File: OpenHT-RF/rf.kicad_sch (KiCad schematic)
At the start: 42 parts, among them J501 EMPCB.CSMAFSTJ.A, J502 Conn_01x02, J503 Conn_01x02, J504 MS300-10F, J505 MS300-10C, SW501 RFSW8008, U501 AT86RF215, X501 ECS-TXO-20CSMV

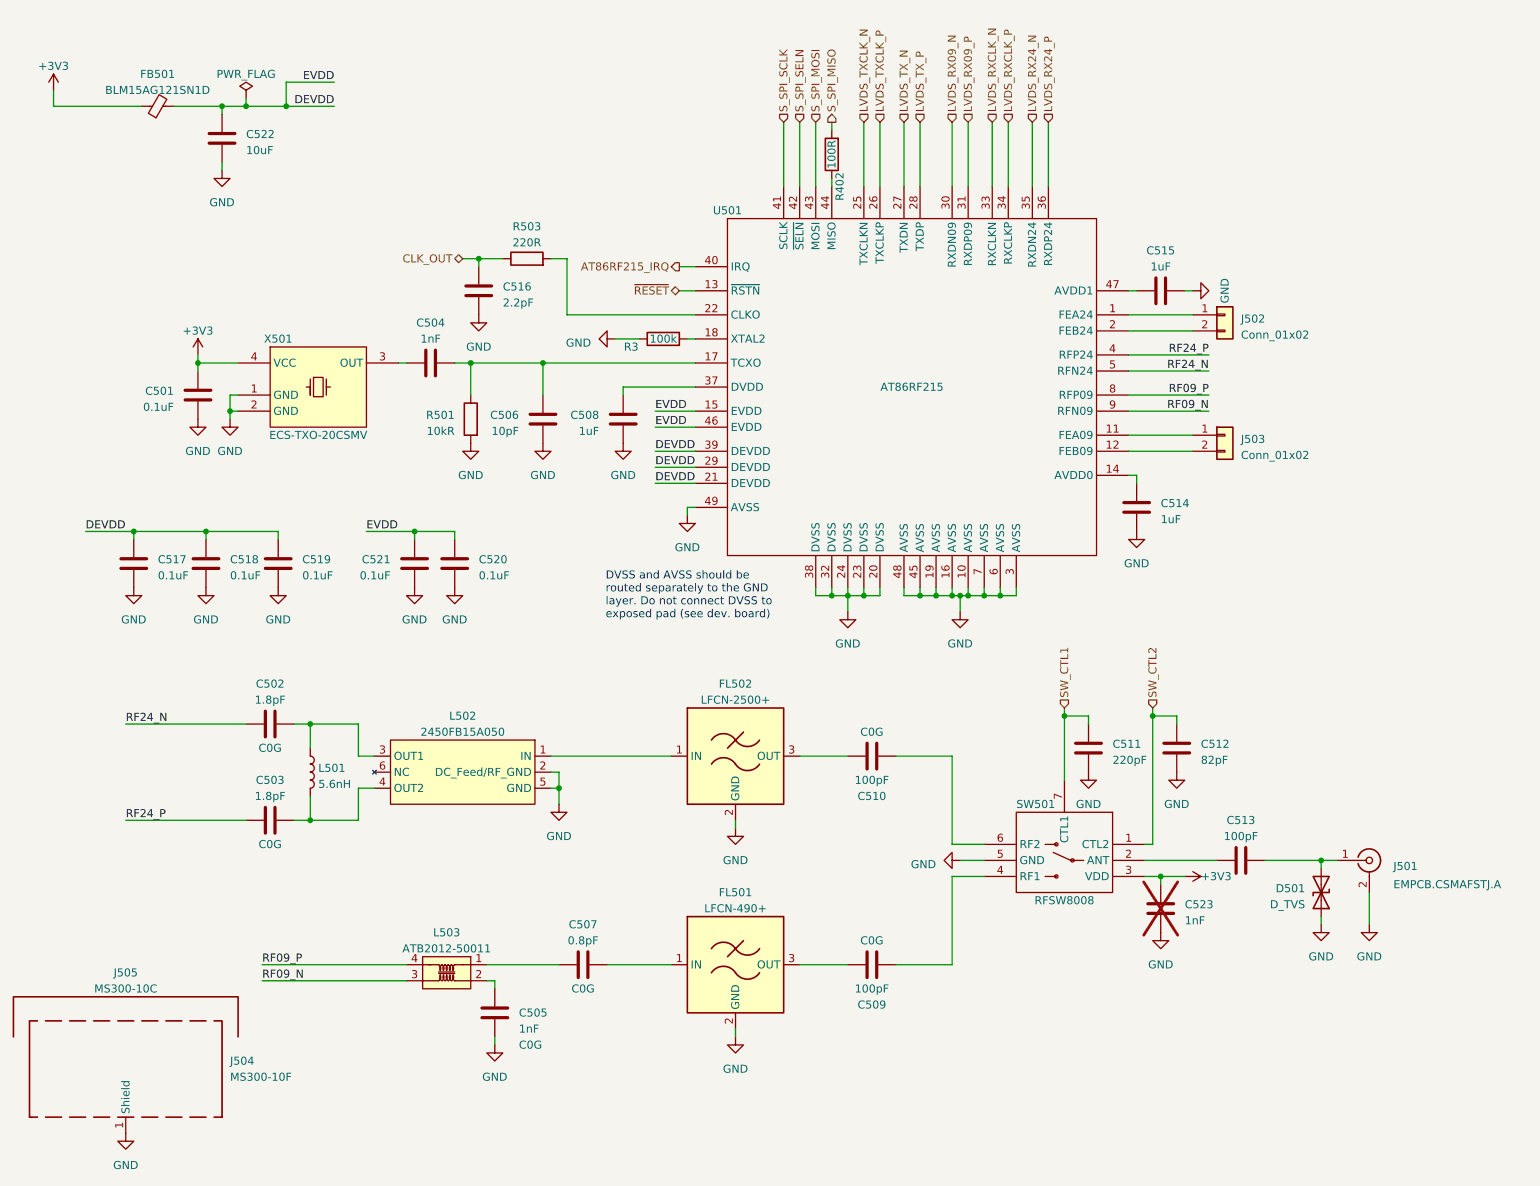
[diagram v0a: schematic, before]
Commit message: Completed components values
Completed dielectric, rated voltage, tolerance, MPN
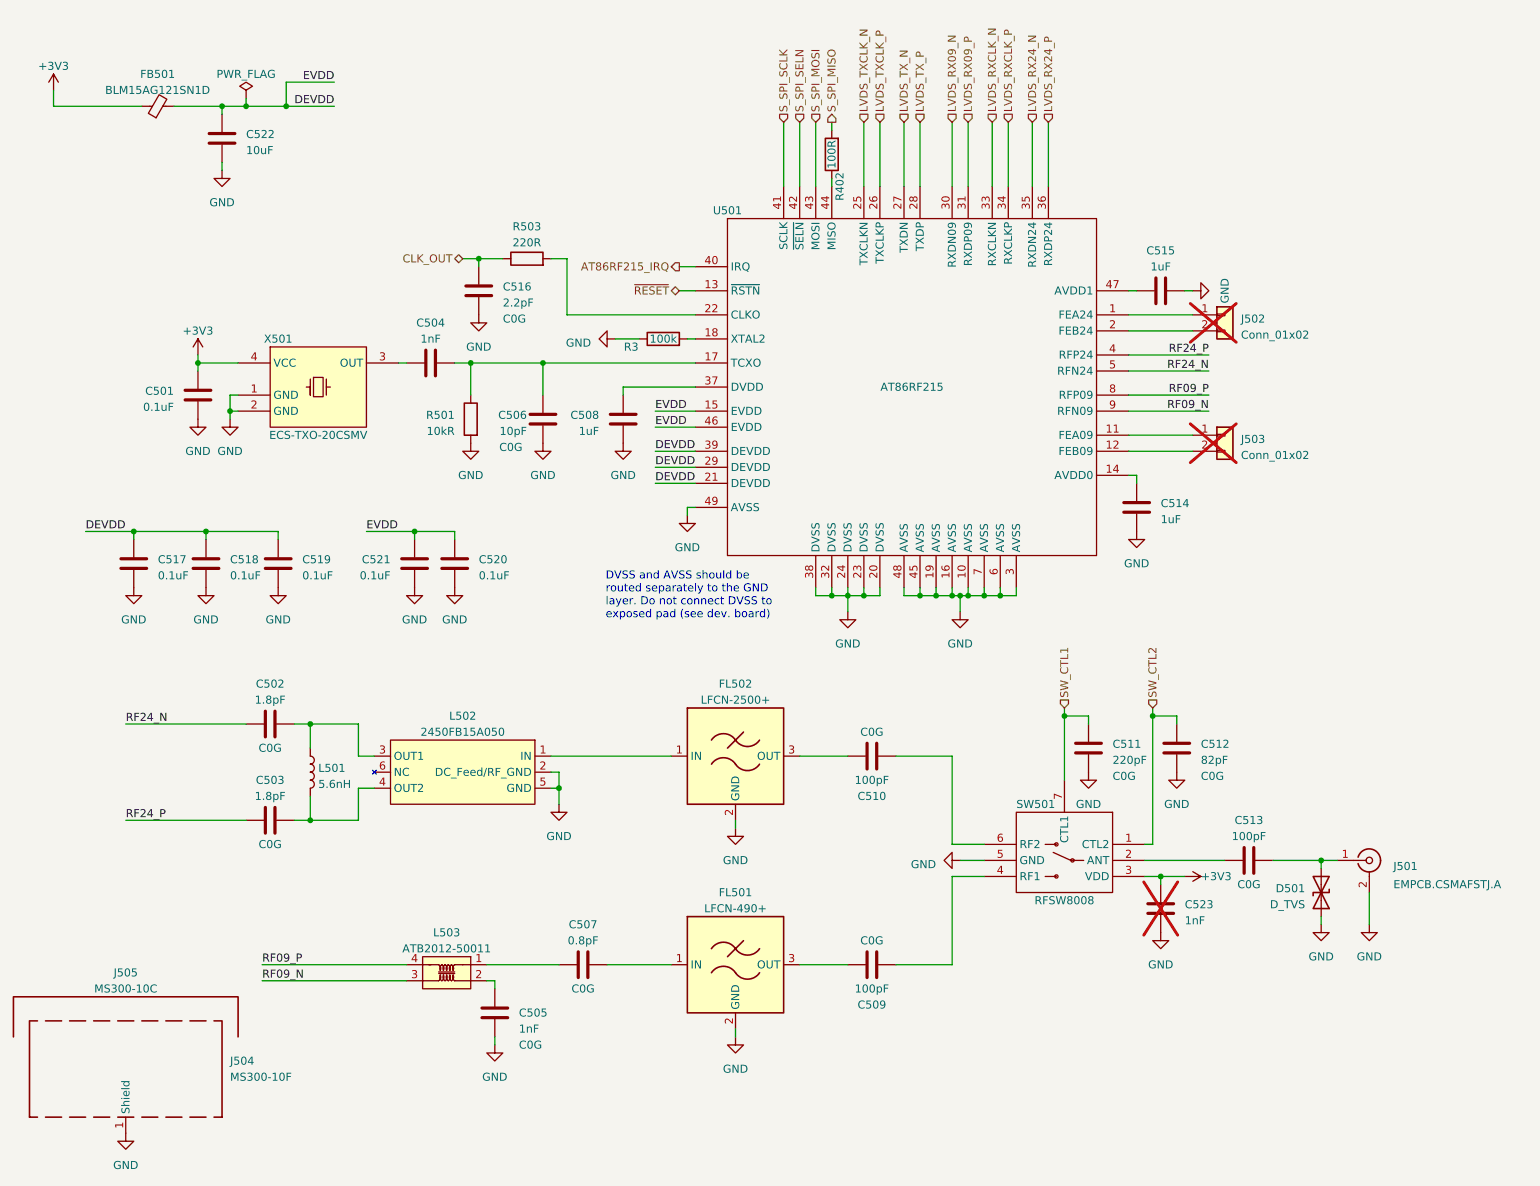
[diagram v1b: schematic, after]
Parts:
- C506, C511, C512, C513, C516: Dielectric (none) -> C0G
- J502, J503: now not fitted
- J505: Manual_Placement (none) -> 1
- R3, R402, R501, R503: Tolerance (none) -> 1%
- SW501: MPN (none) -> RFSW8008TR7
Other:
- moved on the sheet: C513
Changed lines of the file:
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@@
     (stroke (width 0) (type default))
   )
-  (wire (pts (xy 215.9 146.05) (xy 224.79 146.05))
+  (wire (pts (xy 217.17 146.05) (xy 224.79 146.05))
     (stroke (width 0) (type default))
   )
@@
     (stroke (width 0) (type default))
   )
-  (wire (pts (xy 196.85 146.05) (xy 208.28 146.05))
+  (wire (pts (xy 196.85 146.05) (xy 209.55 146.05))
     (stroke (width 0) (type default))
   )
@@
     )
   )
-  (netclass_flag "" (length 2.54) (shape round) (at 217.17 146.05 0) (fields_autoplaced)
+  (netclass_flag "" (length 2.54) (shape round) (at 218.44 146.05 0) (fields_autoplaced)
     (effects (font (size 1.27 1.27)) (justify left bottom))
-    (property "Netclass" "50Ohm" (at 217.8685 143.51 0)
+    (property "Netclass" "50Ohm" (at 219.1385 143.51 0)
       (effects (font (size 1.27 1.27) italic) (justify left))
     )
@@
     )
     (property "MPN" "MS300-10C" (at 35.56 171.45 0)
+      (effects (font (size 1.27 1.27)) hide)
+    )
+    (property "Manual_Placement" "1" (at 35.56 171.45 0)
       (effects (font (size 1.27 1.27)) hide)
     )
@@
       (effects (font (size 1.27 1.27)) hide)
     )
+    (property "Tolerance" "1%" (at 90.17 76.2 0)
+      (effects (font (size 1.27 1.27)) hide)
+    )
     (pin "1")
     (pin "2")
@@
   )
   (symbol (lib_id "Device:C") (at 187.96 128.27 0) (unit 1)
-    (in_bom yes) (on_board yes) (dnp no) (fields_autoplaced)
+    (in_bom yes) (on_board yes) (dnp no)
     (property "Reference" "C511" (at 191.77 127.635 0)
       (effects (font (size 1.27 1.27)) (justify left))
@@
       (effects (font (size 1.27 1.27)) hide)
     )
+    (property "Dielectric" "C0G" (at 191.77 132.715 0)
+      (effects (font (size 1.27 1.27)) (justify left))
+    )
     (pin "1")
     (pin "2")
@@
   )
   (symbol (lib_id "Device:C") (at 201.93 128.27 0) (unit 1)
-    (in_bom yes) (on_board yes) (dnp no) (fields_autoplaced)
+    (in_bom yes) (on_board yes) (dnp no)
     (property "Reference" "C512" (at 205.74 127.635 0)
       (effects (font (size 1.27 1.27)) (justify left))
@@
     (property "Datasheet" "~" (at 201.93 128.27 0)
       (effects (font (size 1.27 1.27)) hide)
+    )
+    (property "Dielectric" "C0G" (at 205.74 132.715 0)
+      (effects (font (size 1.27 1.27)) (justify left))
     )
     (pin "1")
@@
   (symbol (lib_id "Device:C") (at 101.6 76.2 0) (mirror y) (unit 1)
     (in_bom yes) (on_board yes) (dnp no)
-    (property "Reference" "C506" (at 97.79 75.565 0)
-      (effects (font (size 1.27 1.27)) (justify left))
-    )
-    (property "Value" "10pF" (at 97.79 78.105 0)
+    (property "Reference" "C506" (at 99.06 75.565 0)
+      (effects (font (size 1.27 1.27)) (justify left))
+    )
+    (property "Value" "10pF" (at 99.06 78.105 0)
       (effects (font (size 1.27 1.27)) (justify left))
     )
@@
     (property "Datasheet" "~" (at 101.6 76.2 0)
       (effects (font (size 1.27 1.27)) hide)
+    )
+    (property "Dielectric" "C0G" (at 96.52 80.645 0)
+      (effects (font (size 1.27 1.27)))
     )
     (pin "1")
@@
   )
   (symbol (lib_id "Connector_Generic:Conn_01x02") (at 209.55 59.69 0) (unit 1)
-    (in_bom yes) (on_board yes) (dnp no) (fields_autoplaced)
+    (in_bom yes) (on_board yes) (dnp yes) (fields_autoplaced)
     (property "Reference" "J502" (at 212.09 60.325 0)
       (effects (font (size 1.27 1.27)) (justify left))
@@
       (effects (font (size 1.27 1.27)) hide)
     )
+    (property "Tolerance" "1%" (at 120.65 63.5 0)
+      (effects (font (size 1.27 1.27)) hide)
+    )
     (pin "1")
     (pin "2")
@@
       (effects (font (size 1.27 1.27)) hide)
     )
+    (property "Dielectric" "C0G" (at 95.25 60.325 0)
+      (effects (font (size 1.27 1.27)) (justify right))
+    )
     (pin "1")
     (pin "2")
@@
     )
     (property "Datasheet" "~" (at 147.32 34.29 0)
+      (effects (font (size 1.27 1.27)) hide)
+    )
+    (property "Tolerance" "1%" (at 147.32 34.29 90)
       (effects (font (size 1.27 1.27)) hide)
     )
@@
     )
     (property "Datasheet" "https://www.qorvo.com/products/d/da006546" (at 191.77 138.43 0)
+      (effects (font (size 1.27 1.27)) hide)
+    )
+    (property "MPN" "RFSW8008TR7 " (at 191.77 138.43 0)
       (effects (font (size 1.27 1.27)) hide)
     )
@@
       (effects (font (size 1.27 1.27)) hide)
     )
+    (property "Tolerance" "1%" (at 99.06 50.8 90)
+      (effects (font (size 1.27 1.27)) hide)
+    )
     (pin "1")
     (pin "2")
@@
     )
   )
-  (symbol (lib_id "Device:C") (at 212.09 146.05 90) (unit 1)
-    (in_bom yes) (on_board yes) (dnp no) (fields_autoplaced)
-    (property "Reference" "C513" (at 212.09 139.7 90)
-      (effects (font (size 1.27 1.27)))
-    )
-    (property "Value" "100pF" (at 212.09 142.24 90)
-      (effects (font (size 1.27 1.27)))
-    )
-    (property "Footprint" "Capacitor_SMD:C_0402_1005Metric" (at 215.9 145.0848 0)
-      (effects (font (size 1.27 1.27)) hide)
-    )
-    (property "Datasheet" "~" (at 212.09 146.05 0)
-      (effects (font (size 1.27 1.27)) hide)
+  (symbol (lib_id "Device:C") (at 213.36 146.05 90) (unit 1)
+    (in_bom yes) (on_board yes) (dnp no)
+    (property "Reference" "C513" (at 213.36 139.7 90)
+      (effects (font (size 1.27 1.27)))
+    )
+    (property "Value" "100pF" (at 213.36 142.24 90)
+      (effects (font (size 1.27 1.27)))
+    )
+    (property "Footprint" "Capacitor_SMD:C_0402_1005Metric" (at 217.17 145.0848 0)
+      (effects (font (size 1.27 1.27)) hide)
+    )
+    (property "Datasheet" "~" (at 213.36 146.05 0)
+      (effects (font (size 1.27 1.27)) hide)
+    )
+    (property "Dielectric" "C0G" (at 213.36 149.86 90)
+      (effects (font (size 1.27 1.27)))
     )
     (pin "1")
@@
   )
   (symbol (lib_id "Connector_Generic:Conn_01x02") (at 209.55 78.74 0) (unit 1)
-    (in_bom yes) (on_board yes) (dnp no) (fields_autoplaced)
+    (in_bom yes) (on_board yes) (dnp yes) (fields_autoplaced)
     (property "Reference" "J503" (at 212.09 79.375 0)
       (effects (font (size 1.27 1.27)) (justify left))

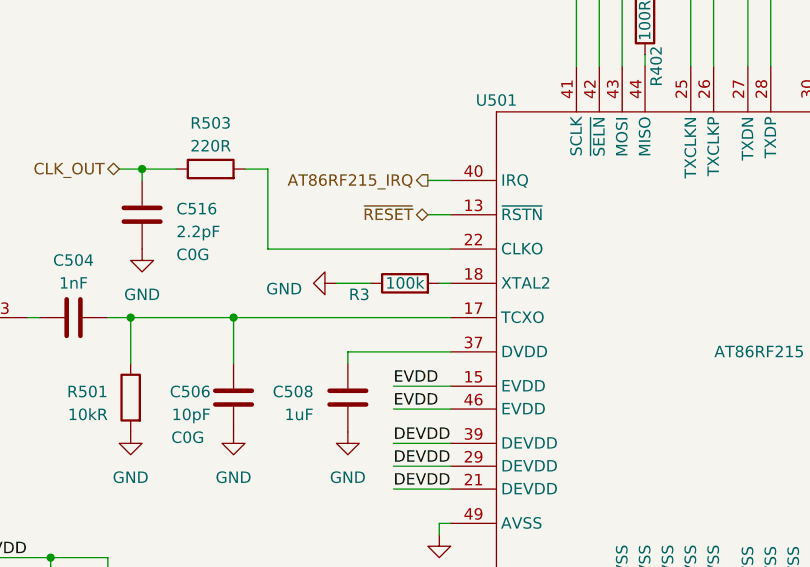
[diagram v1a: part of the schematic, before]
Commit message: Fixed incorrect value for R502
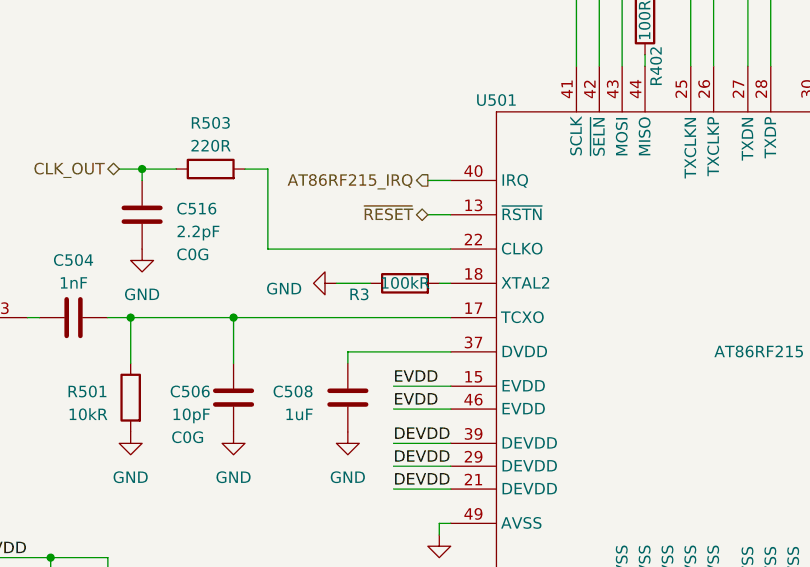
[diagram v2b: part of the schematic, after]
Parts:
- R3: value 100k -> 100kR
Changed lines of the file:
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@@
       (effects (font (size 1.27 1.27)))
     )
-    (property "Value" "100k" (at 120.65 63.5 90)
+    (property "Value" "100kR" (at 120.65 63.5 90)
       (effects (font (size 1.27 1.27)))
     )

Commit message: Added MPN for L501
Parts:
- L501: MPN (none) -> LRC0402CS5N6GV001T
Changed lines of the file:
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@@
+      (effects (font (size 1.27 1.27)) hide)
+    )
+    (property "MPN" "LRC0402CS5N6GV001T" (at 64.77 132.08 0)
       (effects (font (size 1.27 1.27)) hide)
     )
